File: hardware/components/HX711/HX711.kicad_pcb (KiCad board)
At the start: 2 copper layers, 12 parts, among them J1 Conn_01x04, Q1 PNP, U1 HX711

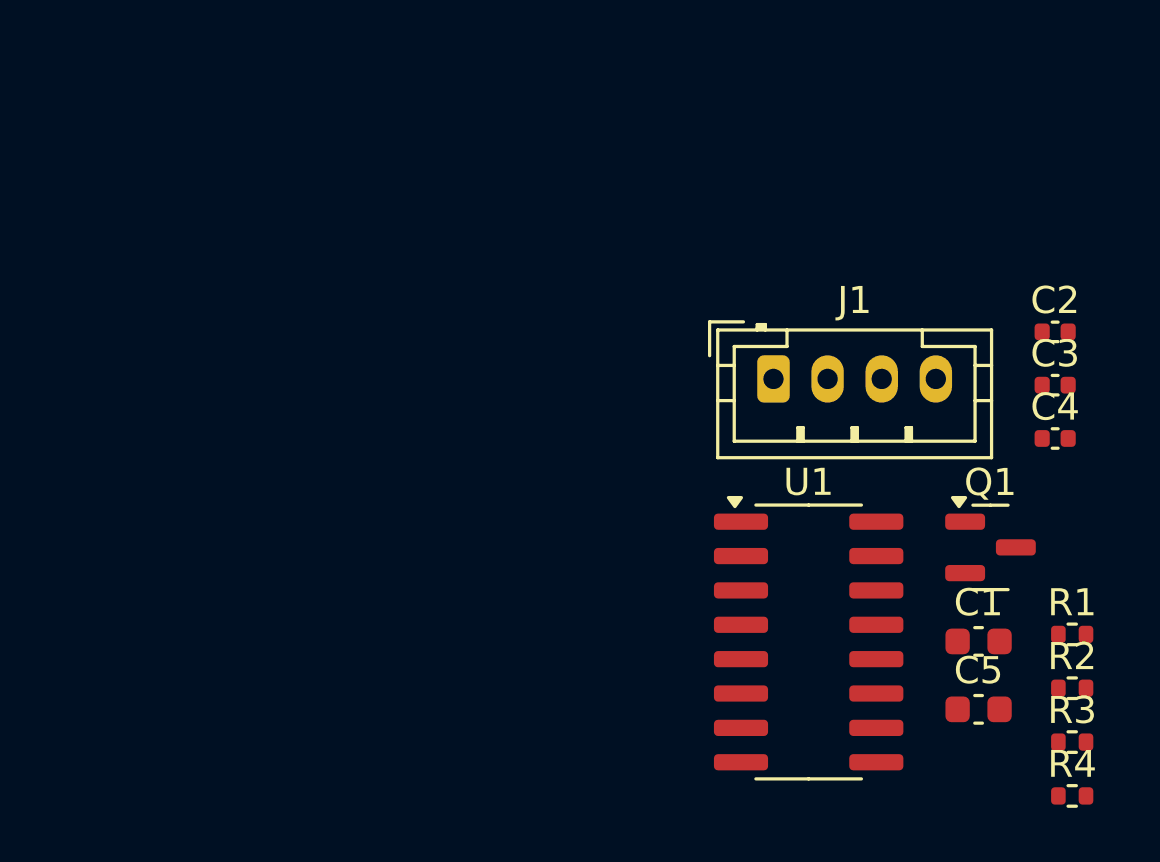
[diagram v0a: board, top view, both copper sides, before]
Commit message: RCS回路作成
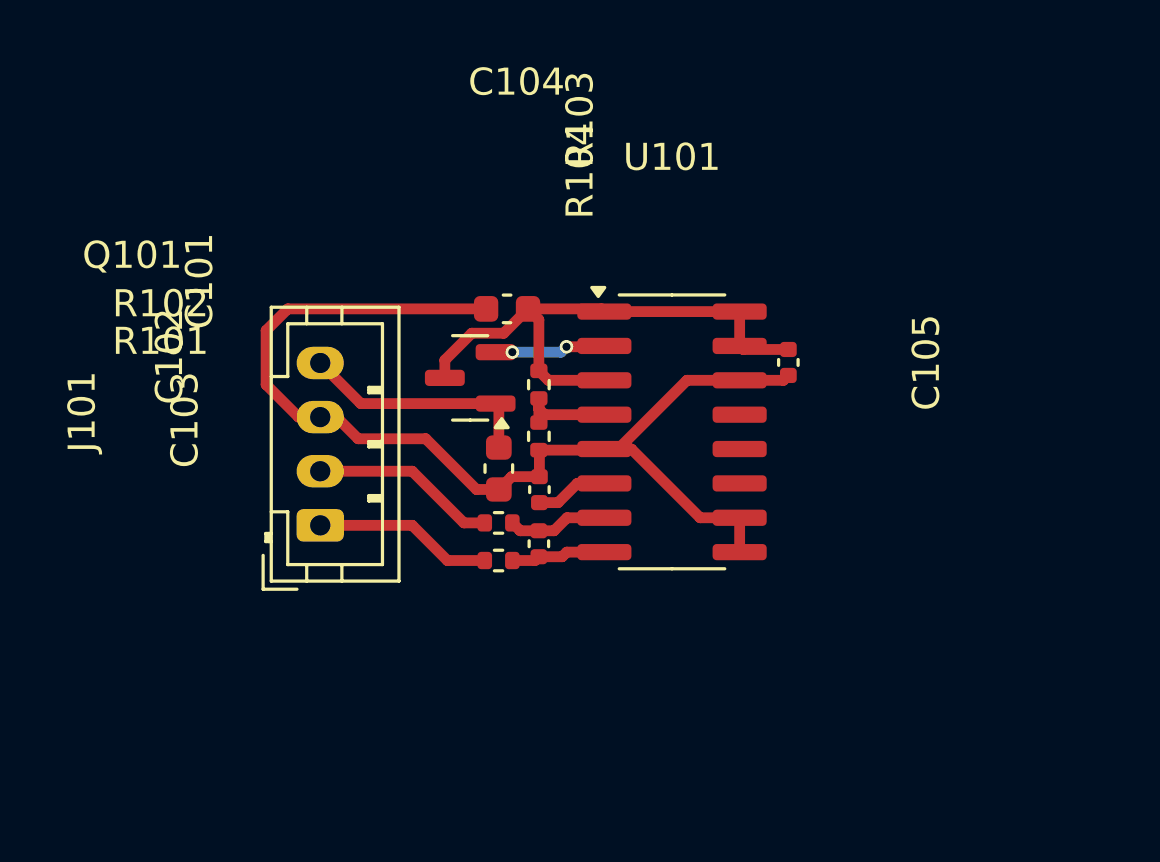
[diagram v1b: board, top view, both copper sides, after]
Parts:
- moved R101 22.9 mm to (141.2, 93.6)
- moved R102 22.7 mm to (141.2, 92.2)
- moved R104 21.8 mm to (142.7, 89.0), turned to -90 degrees
- moved R103 21.8 mm to (142.7, 87.1), turned to -90 degrees
- moved C104 21.3 mm to (141.5, 84.3), turned to 180 degrees
- moved Q101 20.2 mm to (140.1, 86.8), turned to 180 degrees
- moved C103 19.9 mm to (142.7, 91.0), turned to 90 degrees
- moved C101 19.8 mm to (141.2, 90.2), turned to -90 degrees
- moved C102 19.5 mm to (142.7, 93.0), turned to 90 degrees
- moved J101 17.6 mm to (134.6, 92.3), turned to 90 degrees
- moved C105 9.90 mm to (151.9, 86.3), turned to -90 degrees
- moved U101 9.26 mm to (147.6, 88.8)
- renumbered C5 to C101, C4 to C102, C2 to C103, C1 to C104, C3 to C105, J1 to J101, Q1 to Q101, R4 to R101, R3 to R102, R1 to R103, R2 to R104, U1 to U101
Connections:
- J101 pad 1: Net-(J1-Pin_1) -> Net-(J101-Pin_1)
- J101 pad 2: Net-(J1-Pin_2) -> Net-(J101-Pin_2)
- R101 pad 1: Net-(J1-Pin_2) -> Net-(J101-Pin_1)
- R102 pad 1: Net-(J1-Pin_1) -> Net-(J101-Pin_2)
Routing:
- net GND: track 0.00 -> 41.0 mm
- net VDD: track 0.00 -> 20.5 mm
- net Net-(J101-Pin_4): track 0.00 -> 8.78 mm
- net Net-(J101-Pin_2): track 0.00 -> 6.87 mm
- net Net-(J101-Pin_1): track 0.00 -> 6.62 mm
- net Net-(Q101-B): track 0.00 -> 4.12 mm, vias 0 -> 2
- net Net-(U101-VFB): track 0.00 -> 3.79 mm
- net Net-(U101-INA-): track 0.00 -> 3.72 mm
- net Net-(U101-INA+): track 0.00 -> 3.53 mm
- net Net-(U101-VBG): track 0.00 -> 2.69 mm
